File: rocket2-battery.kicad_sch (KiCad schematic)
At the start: 1 part

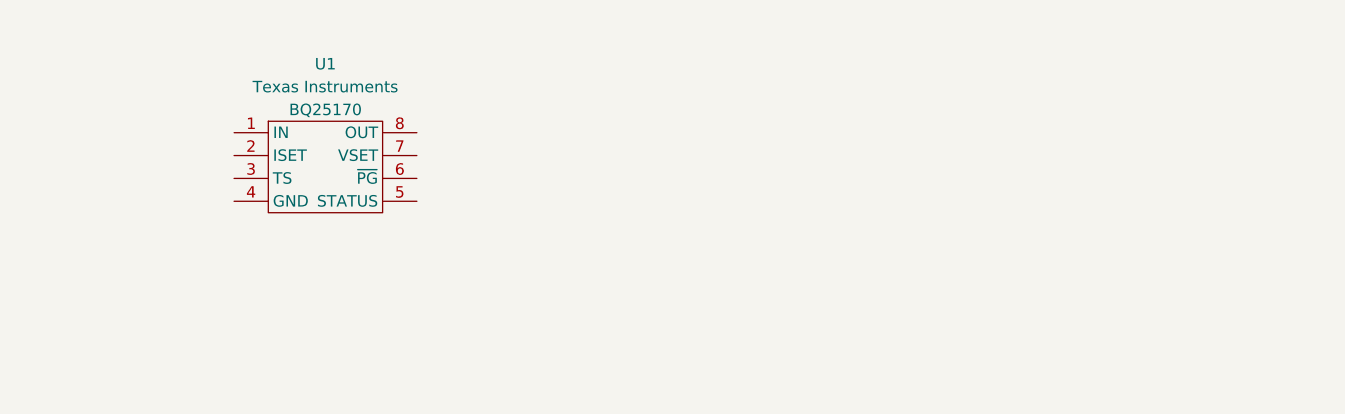
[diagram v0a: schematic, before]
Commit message: Basic schematic
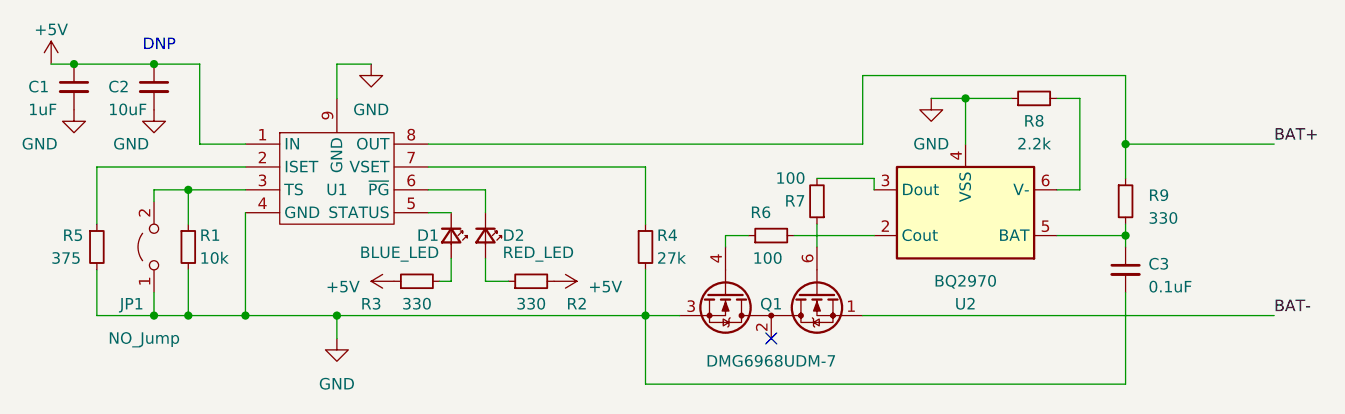
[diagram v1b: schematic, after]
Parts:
- added C1: 1uF, symbol Device:C_Small
- added C2: 10uF, symbol Device:C_Small
- added C3: 0.1uF, symbol Device:C_Small
- added D1: BLUE_LED, symbol Device:LED_Small
- added D2: RED_LED, symbol Device:LED_Small
- added JP1: NO_Jump, symbol Jumper:Jumper_2_Open
- added Q1: DMG6968UDM-7, Package_TO_SOT_SMD:SOT-23-6, symbol Transistor_FET:DMG9926UDM
- added R1: 10k, symbol Device:R_Small
- added R2, R3, R9: 330, symbol Device:R_Small
- added R4: 27k, symbol Device:R_Small
- added R5: 375, symbol Device:R_Small
- added R6, R7: 100, symbol Device:R_Small
- added R8: 2.2k, symbol Device:R_Small
- added U2: BQ2970, Package_SON:WSON-6_1.5x1.5mm_P0.5mm, symbol Battery_Management:BQ297xy
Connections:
- net +5V: now reaches U1.1 (IN)
- net +5V: now also C1.1, C2.1, R2.2, R3.1
- net at U1.2 (ISET): now also R5.1
- net at U1.3 (TS): now also JP1.2 (B), R1.1
- net GND: now reaches U1.4 (GND)
- net GND: now also U1.9 (GND), C1.2, C2.2, C3.2, JP1.1 (A), Q1.3 (S2), R1.2, R4.2, R5.2, R8.1, U2.4 (VSS)
- net at U1.5 (STATUS): now also D1.1 (K)
- net at U1.6 (~{PG}): now also D2.1 (K)
- net at U1.7 (VSET): now also R4.1
- net BAT+: now reaches U1.8 (OUT)
- net BAT+: now also R9.1
- new net: Q1.2 (S1/D2), Q1.5 (S1/D2)
- new net: Q1.4 (G2), R6.1
- new net: Q1.6 (G1), R7.1
- new net: R7.2, U2.3 (Dout)
- new net: D2.2 (A), R2.1
- new net: R6.2, U2.2 (Cout)
- new net: D1.2 (A), R3.2
- new net: C3.1, R9.2, U2.5 (BAT)
- new net: R8.2, U2.6 (V-)
- new net BAT-: Q1.1 (D1)
- no-connect marks 0 -> 1
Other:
- note added: "DNP"
